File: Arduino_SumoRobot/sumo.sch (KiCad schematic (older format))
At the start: 54 parts, among them IC1 40106D, K1 RELAY_C, K2 RELAY_C, K3 RELAY_C, K4 RELAY_C, P1 Power, P10 CONN_01X04, P11 CONN_01X04, P12 CONN_01X02, P13 CONN_01X04, P14 CONN_01X04, P15 CONN_01X04, P16 CONN_01X04, P17 CONN_01X02, P18 CONN_01X02, P2 Analog, P3 Digital, P4 Digital, P5 CONN_1, P6 CONN_1, P7 CONN_1, P8 CONN_1, P9 CONN_01X06, Q1 S8050, Q2 S8050, Q3 S8050, Q4 S8050

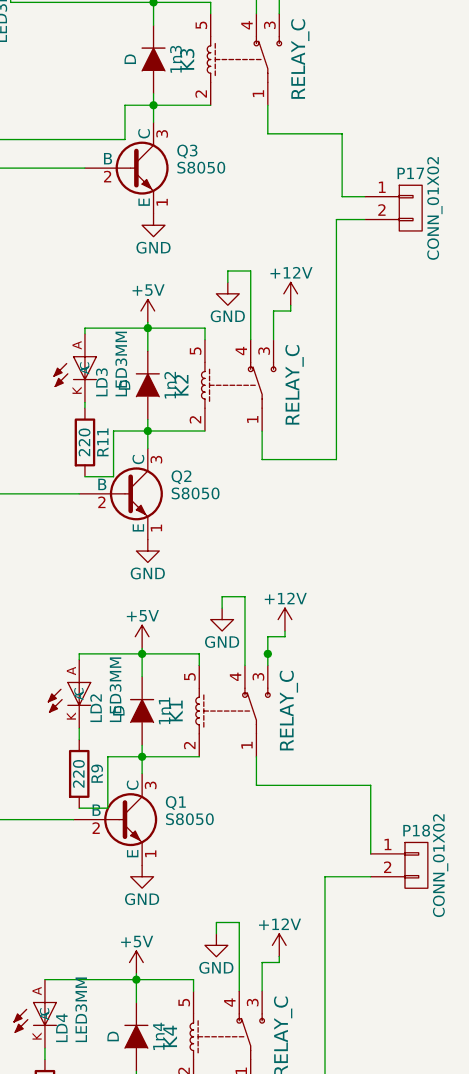
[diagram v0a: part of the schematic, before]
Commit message: Correcciones varias, serigrafía, ruteo, borneras, puentes, planos, etc.
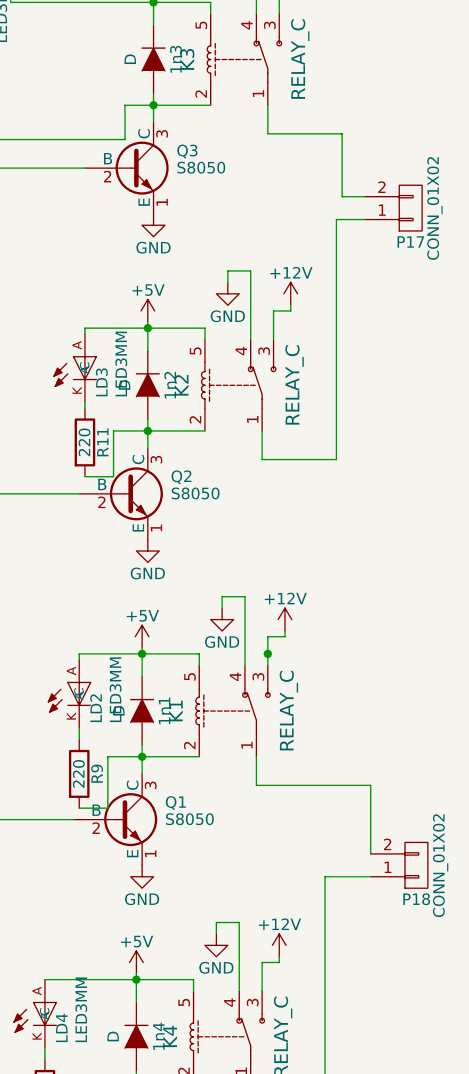
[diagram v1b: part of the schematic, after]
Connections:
- net at K4.1: now also P18.1 (P1); no longer P18.2 (P2)
- net at K1.1: now also P18.2 (P2); no longer P18.1 (P1)
- net at K2.1: now also P17.1 (P1); no longer P17.2 (P2)
- net at K3.1: now also P17.2 (P2); no longer P17.1 (P1)
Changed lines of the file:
@@
 F 3 "" H 11000 4875 50  0000 C CNN
 	1    11000 4875
-	1    0    0    -1
+	1    0    0    1
 $EndComp
 $Comp
@@
 F 3 "" H 10975 2000 50  0000 C CNN
 	1    10975 2000
-	1    0    0    -1
+	1    0    0    1
 $EndComp
 $Comp
